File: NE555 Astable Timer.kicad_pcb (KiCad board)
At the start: 2 copper layers, 38 x 30 mm, 8 parts, among them J1 Conn_01x02_Pin, U1 LM555xM

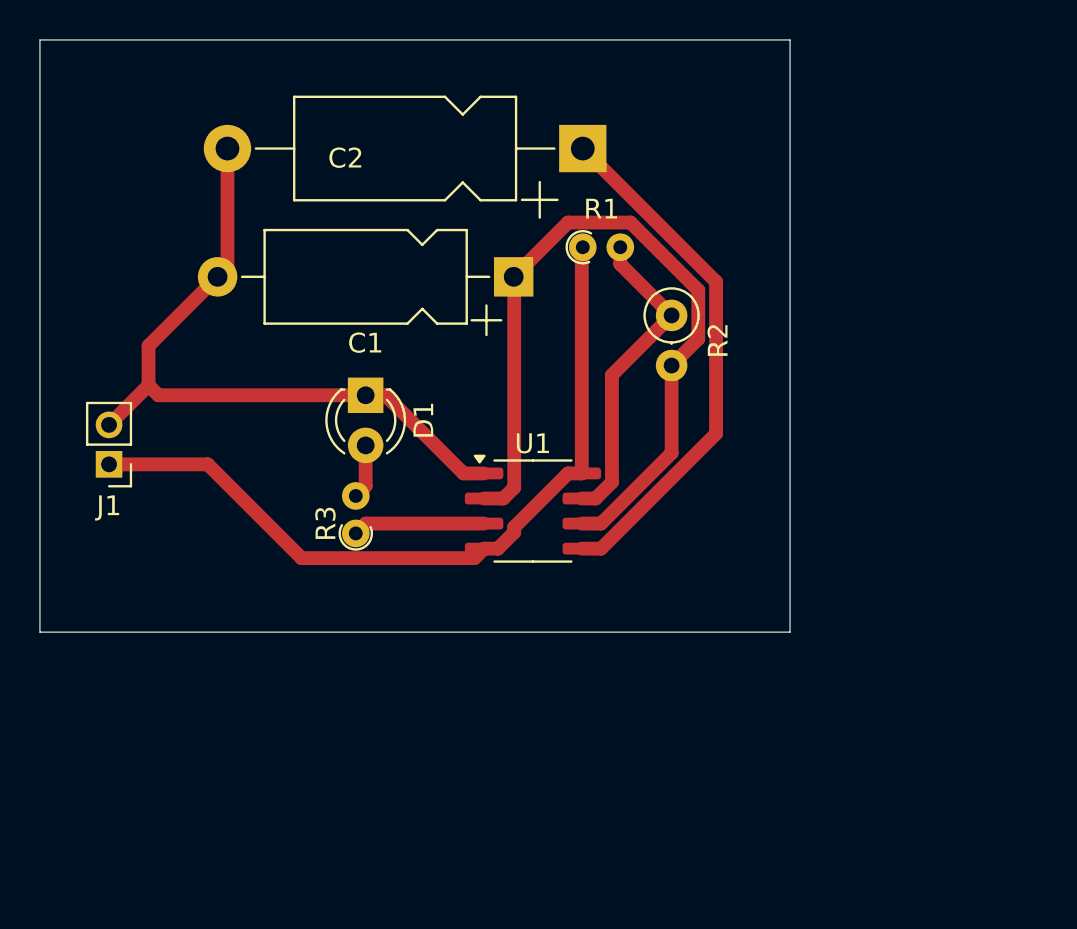
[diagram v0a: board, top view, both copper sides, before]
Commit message: potentiometer update
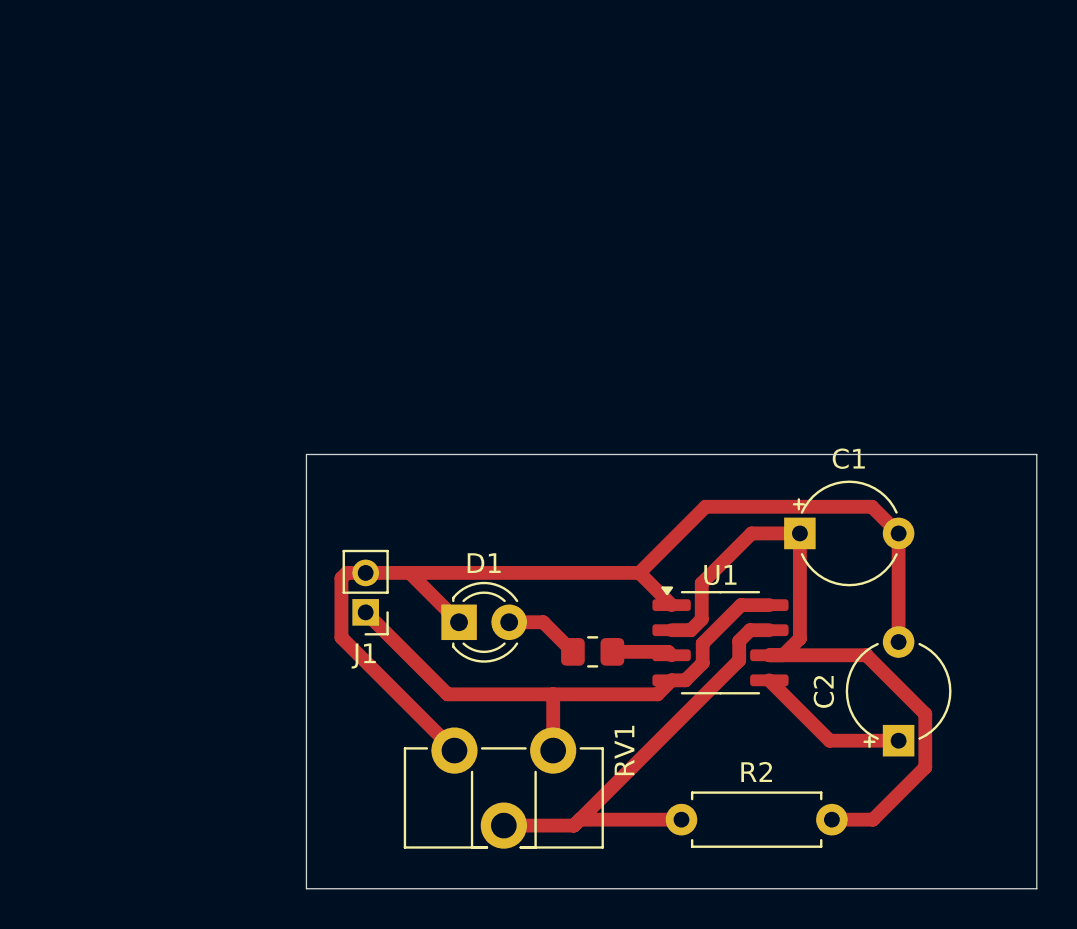
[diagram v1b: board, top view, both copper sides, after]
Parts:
- removed R1: R, Resistor_THT:R_Axial_DIN0204_L3.6mm_D1.6mm_P1.90mm_Vertical
- added RV1: R_Potentiometer, Potentiometer_THT:Potentiometer_ACP_CA9-H3,8_Horizontal, F.Cu at (134.5, 115.5)
- C1: footprint Capacitor_THT:CP_Axial_L10.0mm_D4.5mm_P15.00mm_Horizontal -> Capacitor_THT:CP_Radial_Tantal_D5.0mm_P5.00mm
- C2: footprint Capacitor_THT:CP_Axial_L11.0mm_D5.0mm_P18.00mm_Horizontal -> Capacitor_THT:CP_Radial_Tantal_D5.0mm_P5.00mm
- R2: footprint Resistor_THT:R_Axial_DIN0207_L6.3mm_D2.5mm_P2.54mm_Vertical -> Resistor_THT:R_Axial_DIN0207_L6.3mm_D2.5mm_P7.62mm_Horizontal
- R3: footprint Resistor_THT:R_Axial_DIN0204_L3.6mm_D1.6mm_P1.90mm_Vertical -> Resistor_SMD:R_0805_2012Metric_Pad1.20x1.40mm_HandSolder
- moved C2 34.0 mm to (152.0, 115.0), turned to 90 degrees
- moved R2 25.5 mm to (141.0, 119.0), turned to 0 degrees
- moved C1 19.5 mm to (147.0, 104.5), turned to 0 degrees
- moved J1 15.0 mm to (125.0, 108.5)
- moved R3 13.4 mm to (136.5, 110.5), turned to 180 degrees
- moved D1 12.4 mm to (129.7, 109.0), turned to 0 degrees
- moved U1 11.6 mm to (143.0, 110.0)
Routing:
- net Net-(U1-CV): track 26.5 -> 7.82 mm
- net GND: track 35.3 -> 52.7 mm
- net VCC: track 39.3 -> 27.5 mm
- net Net-(U1-DIS): track 16.1 -> 23.7 mm
- net Net-(U1-THR): track 39.2 -> 34.5 mm
- net Net-(U1-Q): track 6.71 -> 3.07 mm
- net Net-(D1-A): track 2.77 -> 3.85 mm
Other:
- board size 38 x 30 mm -> 37 x 22 mm
